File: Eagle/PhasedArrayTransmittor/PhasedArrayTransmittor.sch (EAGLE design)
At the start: 71 parts, among them IC1 OP400P, IC2 LM555D, IC3 LM555D, IC4 LM555D, IC5 LM555D

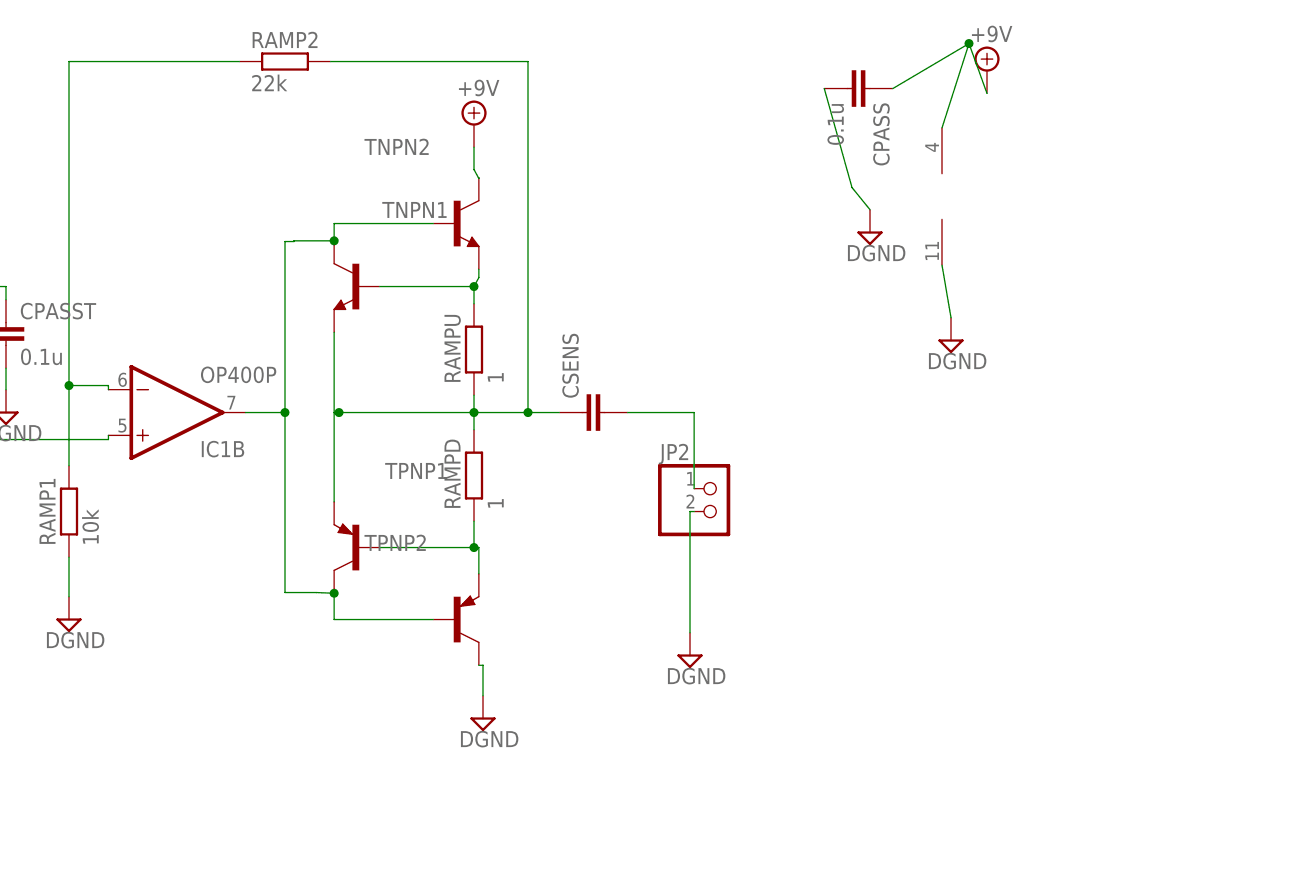
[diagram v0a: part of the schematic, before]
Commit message: Add files via upload
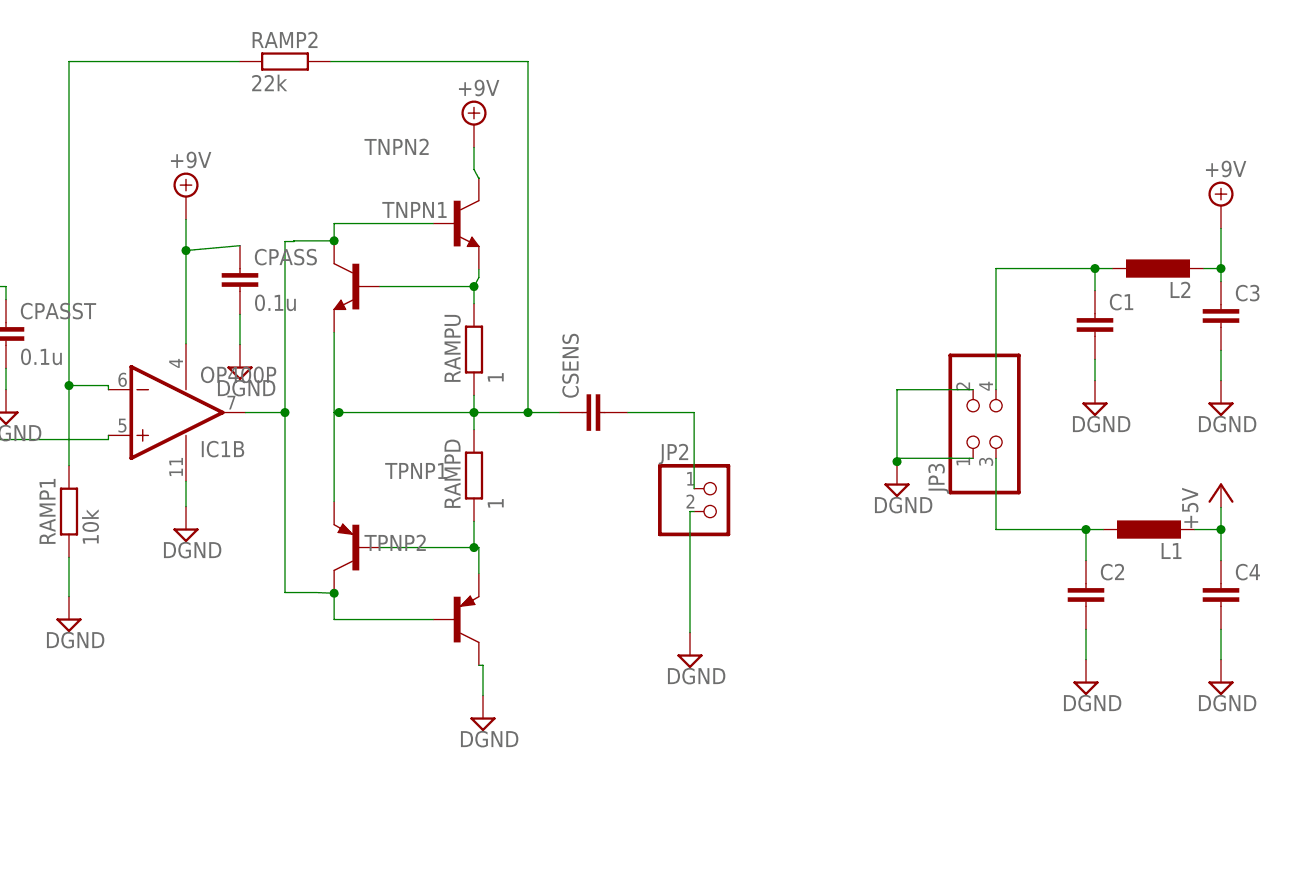
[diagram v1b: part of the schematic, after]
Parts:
- added C1, C2, C3, C4: (no value), rcl:C-EU025-024X044
- added JP3: (no value), pinhead:PINHD-2X2
- added L1, L2: (no value), rcl:L-EU0207/7
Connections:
- new net N$49: C2.1, JP3.3, L1.1
- new net N$51: C1.1, JP3.4, L2.1
- net +5V: now also C4.1, L1.2
- net +9V: now also C3.1, L2.2
- net DGND: now also C1.2, C2.2, C3.2, C4.2, JP3.1, JP3.2
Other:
- moved on the sheet: CPASS
